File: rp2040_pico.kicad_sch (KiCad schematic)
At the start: 1 part, among them U1 Pico

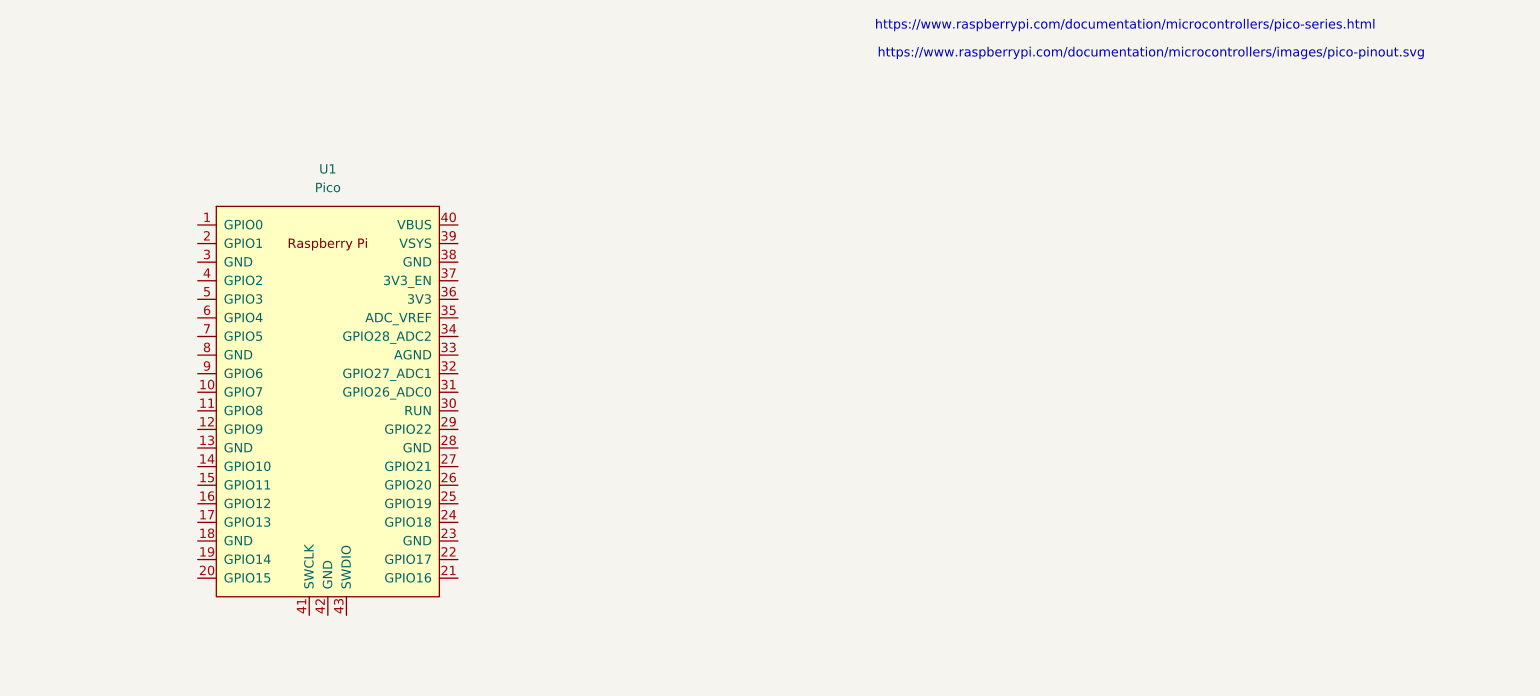
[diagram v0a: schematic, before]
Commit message: update design
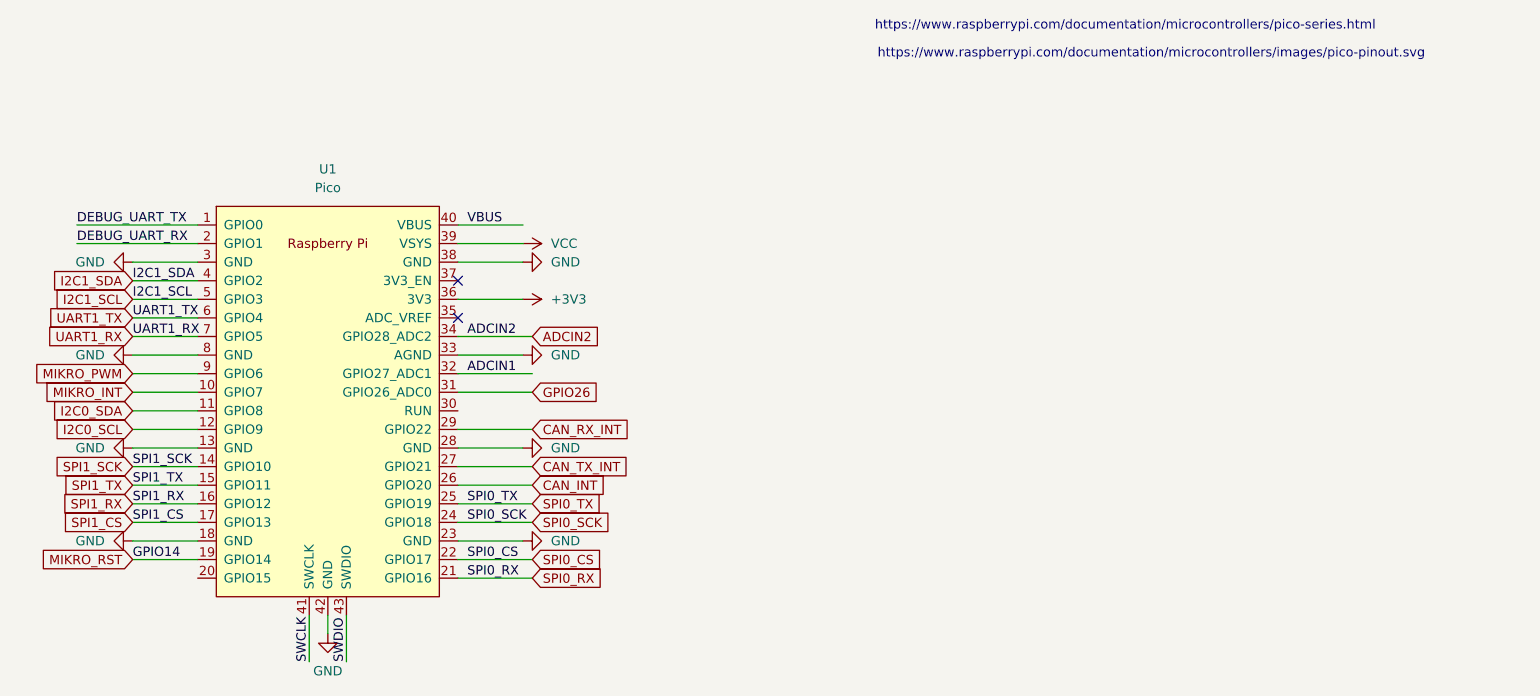
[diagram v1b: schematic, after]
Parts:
- U1: footprint RPi_Pico:RPi_Pico_SMD_TH -> rpi-pico:RPi_Pico_SMD_TH
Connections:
- net DEBUG_UART_TX: now reaches U1.1 (GPIO0)
- net MIKRO_INT: now reaches U1.10 (GPIO7)
- net I2C0_SDA: now reaches U1.11 (GPIO8)
- net I2C0_SCL: now reaches U1.12 (GPIO9)
- net GND: now reaches U1.13 (GND)
- net GND: now also U1.18 (GND), U1.23 (GND), U1.28 (GND), U1.3 (GND), U1.33 (AGND), U1.38 (GND), U1.42 (GND), U1.8 (GND)
- net SPI1_SCK: now reaches U1.14 (GPIO10)
- net SPI1_TX: now reaches U1.15 (GPIO11)
- net SPI1_RX: now reaches U1.16 (GPIO12)
- net SPI1_CS: now reaches U1.17 (GPIO13)
- net MIKRO_RST: now reaches U1.19 (GPIO14)
- net DEBUG_UART_RX: now reaches U1.2 (GPIO1)
- net SPI0_RX: now reaches U1.21 (GPIO16)
- net SPI0_CS: now reaches U1.22 (GPIO17)
- net SPI0_SCK: now reaches U1.24 (GPIO18)
- net SPI0_TX: now reaches U1.25 (GPIO19)
- net CAN_INT: now reaches U1.26 (GPIO20)
- net CAN_TX_INT: now reaches U1.27 (GPIO21)
- net CAN_RX_INT: now reaches U1.29 (GPIO22)
- net GPIO26: now reaches U1.31 (GPIO26_ADC0)
- net ADCIN1: now reaches U1.32 (GPIO27_ADC1)
- net ADCIN2: now reaches U1.34 (GPIO28_ADC2)
- net +3V3: now reaches U1.36 (3V3)
- net VCC: now reaches U1.39 (VSYS)
- net I2C1_SDA: now reaches U1.4 (GPIO2)
- net VBUS: now reaches U1.40 (VBUS)
- net SWCLK: now reaches U1.41 (SWCLK)
- net SWDIO: now reaches U1.43 (SWDIO)
- net I2C1_SCL: now reaches U1.5 (GPIO3)
- net UART1_TX: now reaches U1.6 (GPIO4)
- net UART1_RX: now reaches U1.7 (GPIO5)
- net MIKRO_PWM: now reaches U1.9 (GPIO6)
- no-connect marks 0 -> 2
